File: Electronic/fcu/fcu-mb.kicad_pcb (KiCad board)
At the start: 2 copper layers, 114.3 x 71.1 mm, 48 parts, among them U1 MAX7219, U101 Connector-FPC-50pins, U2 MAX7219, U3 MAX7219

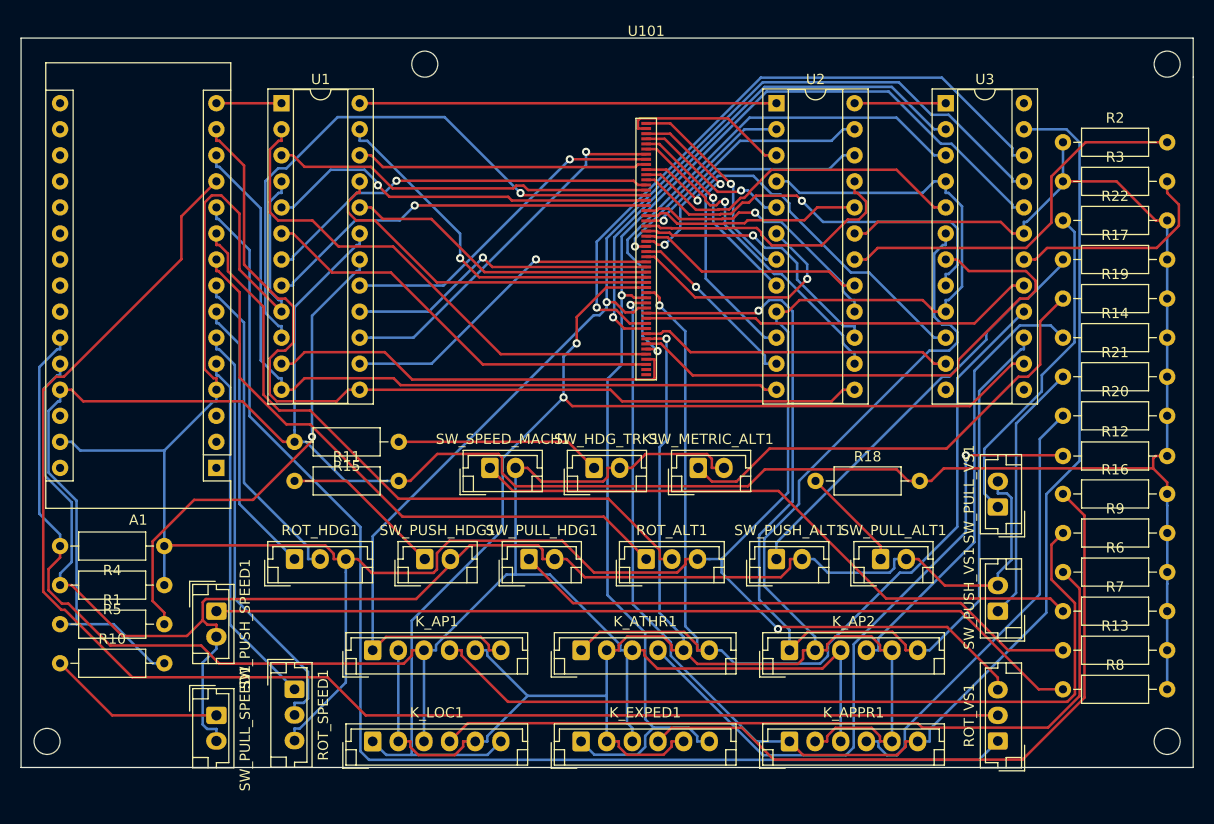
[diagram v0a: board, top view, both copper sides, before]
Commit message: Update fcu schemas and libraries
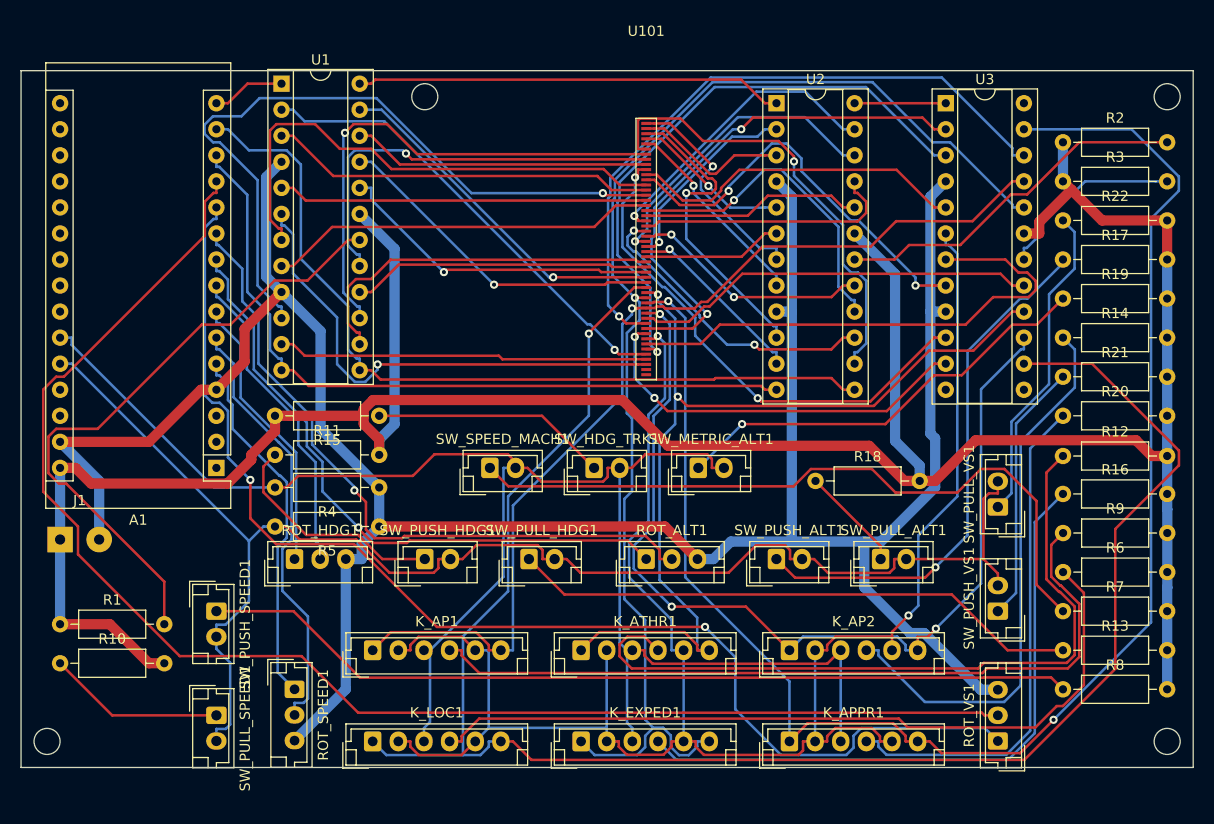
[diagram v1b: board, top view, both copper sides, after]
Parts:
- added J1: Conn_Coaxial_Power, Connector_Wire:SolderWirePad_1x02_P3.81mm_Drill1mm, F.Cu at (52.1, 123.8)
- moved R4 21.7 mm to (83.2, 118.7)
- moved R5 21.7 mm to (83.2, 122.6)
- moved R11 3.18 mm to (73.0, 115.6)
- moved R15 3.17 mm to (83.2, 111.8)
- moved U1 1.91 mm to (73.7, 79.4)
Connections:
- A1 pad 27: +5V -> Net-(A1-Pad27)
- A1 pad 30: Net-(A1-Pad30) -> +5V
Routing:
- net Dr3SegA: track 117.9 -> 174.4 mm, vias 2 -> 1
- net Dr3SegE: track 119.4 -> 97.1 mm
- net Dr3SegD: track 138.0 -> 154.5 mm, vias 1 -> 2
- net GND: track 271.1 -> 256.0 mm, vias 1 -> 0
- net Dr3SegB: track 107.4 -> 92.4 mm, vias 1 -> 2
- net Net-(R1-Pad2): track 47.9 -> 61.7 mm, vias 1 -> 0
- net speedAltF: track 36.3 -> 49.9 mm
- net BTN_GRP_2: track 154.8 -> 141.5 mm
- net hdgVsA: track 31.9 -> 44.6 mm
- net Dr3Dig5: track 38.7 -> 50.4 mm, vias 1 -> 2
- net speedAltDig3: track 39.1 -> 50.7 mm, vias 1 -> 0
- net speedAltDig5: track 59.0 -> 70.6 mm
- net Net-(K_AP2-Pad4): track 43.3 -> 54.7 mm
- net Net-(R17-Pad1): track 41.6 -> 52.3 mm, vias 0 -> 1
- net BTN_GRP_1: track 177.3 -> 166.8 mm
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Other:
- board size 114.3 x 71.1 mm -> 114.3 x 67.9 mm
